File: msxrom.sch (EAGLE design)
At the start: 9 parts

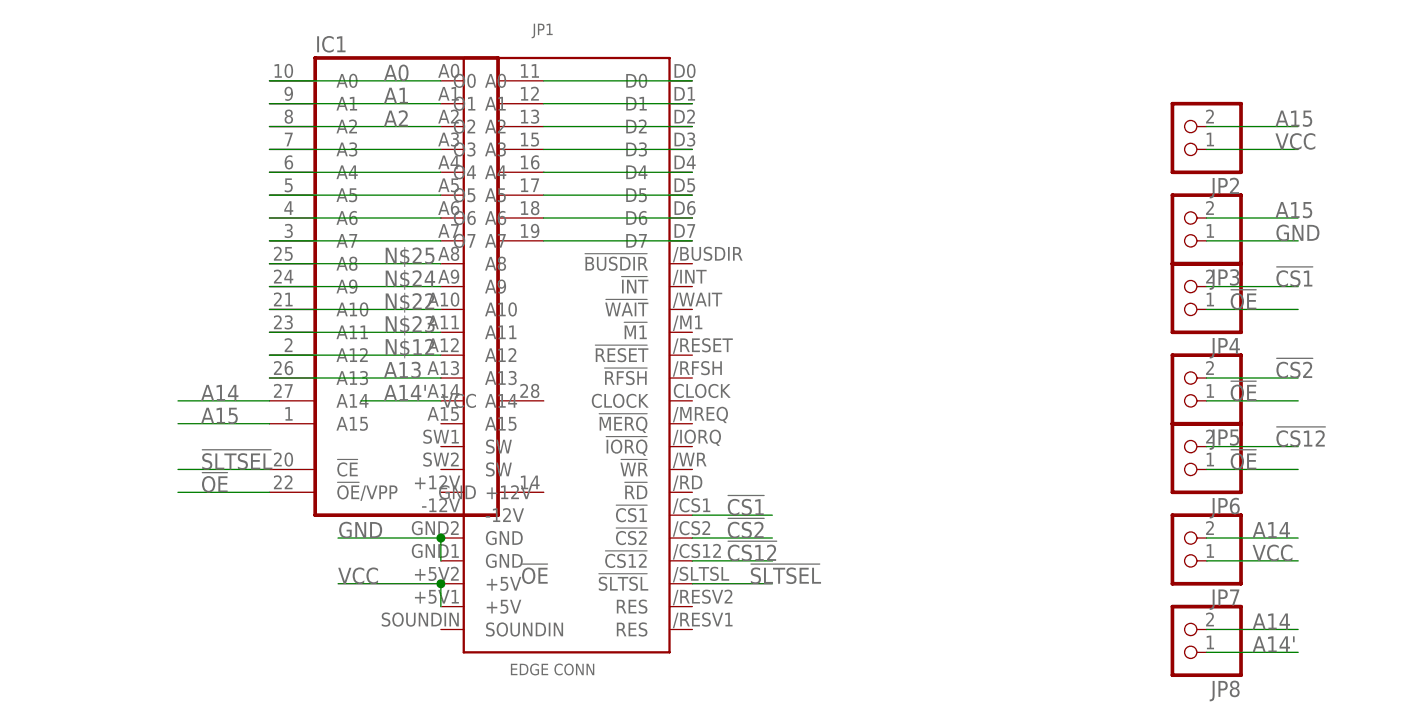
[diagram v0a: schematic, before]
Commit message: with io breakout
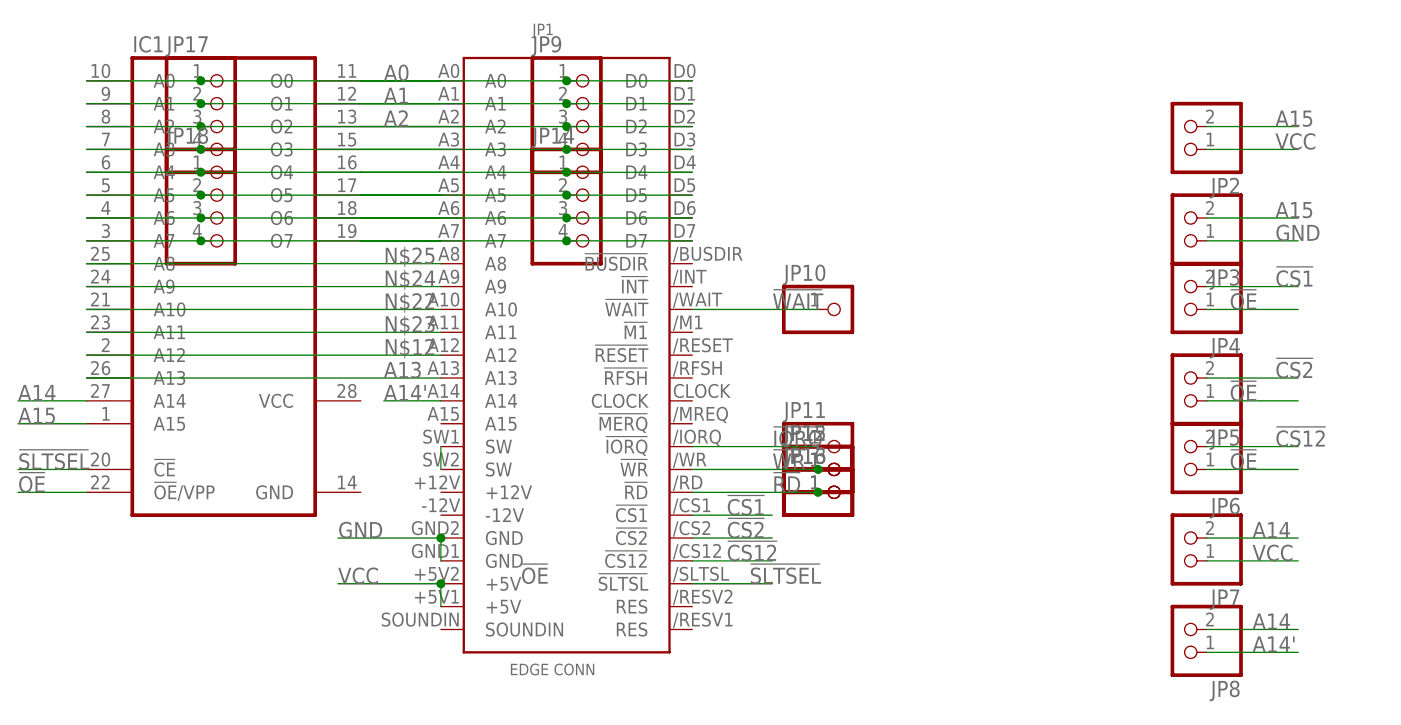
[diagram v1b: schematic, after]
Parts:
- added JP10, JP11, JP12, JP13, JP15, JP16: (no value), pinhead-round:PINHD-1X1
- added JP14, JP17, JP18, JP9: (no value), pinhead-round:PINHD-1X4
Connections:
- new net !IORQ: JP1.!IORQ, JP11.1
- new net !RD: JP1.!RD, JP13.1, JP16.1
- new net !WAIT: JP1.!WAIT, JP10.1
- new net !WR: JP1.!WR, JP12.1, JP15.1
- new net N$9: JP1.SW@1, JP1.SW@2
- net A0: now also JP17.1
- net A1: now also JP17.2
- net A2: now also JP17.3
- net N$1: now also JP9.1
- net N$13: now also JP18.4
- net N$14: now also JP18.3
- net N$15: now also JP18.2
- net N$16: now also JP18.1
- net N$17: now also JP17.4
- net N$2: now also JP9.2
- net N$3: now also JP9.3
- net N$4: now also JP9.4
- net N$5: now also JP14.1
- net N$6: now also JP14.2
- net N$7: now also JP14.3
- net N$8: now also JP14.4
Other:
- moved on the sheet: IC1
